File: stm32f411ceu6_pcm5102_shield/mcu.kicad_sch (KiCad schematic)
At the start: 25 parts, among them J100 Conn_01x04_Pin, J101 Conn_01x04_Pin, SW100 RotaryEncoder_Switch_MP, U100 BlackPill, U101 INMP411

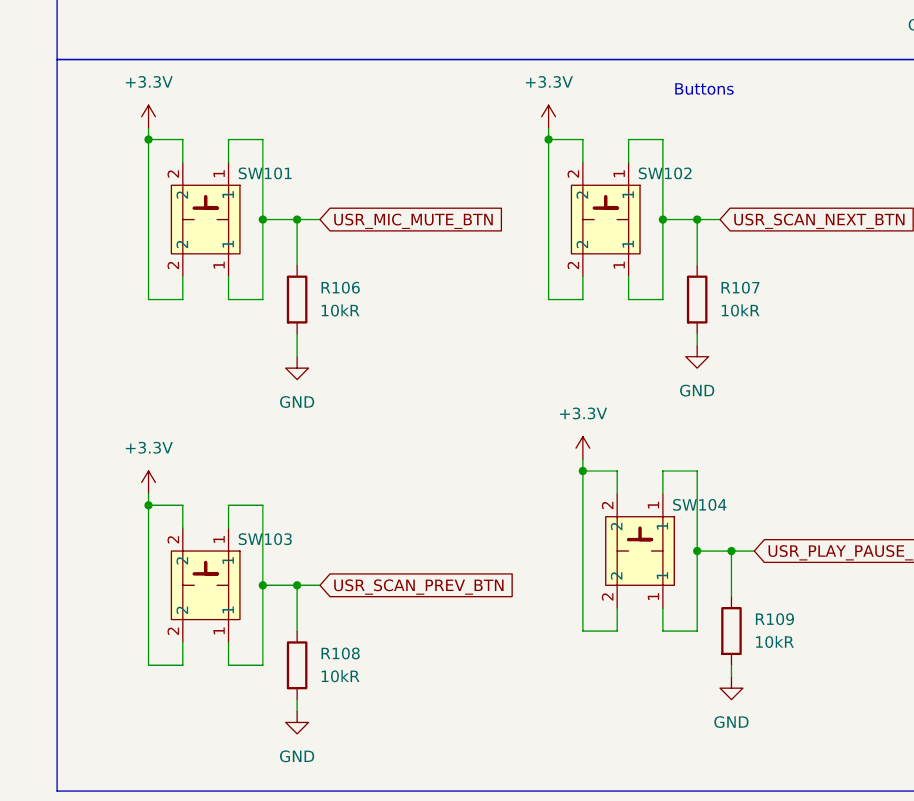
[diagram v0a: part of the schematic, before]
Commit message: Put all items on a board
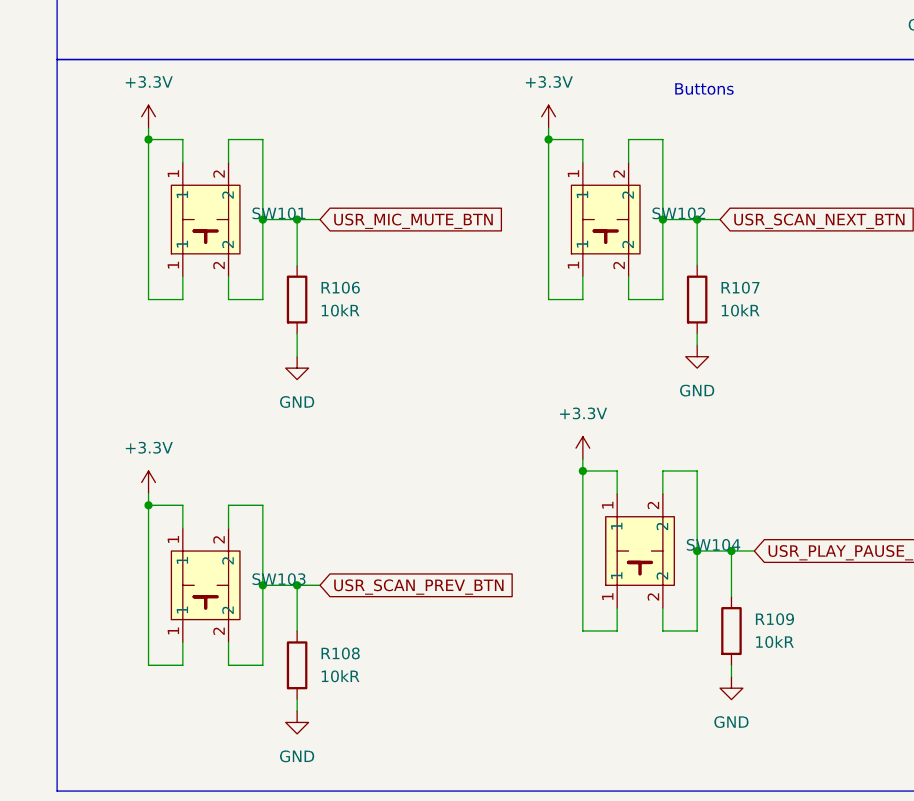
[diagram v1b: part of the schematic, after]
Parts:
- removed SW101, SW102, SW103, SW104: ~, Button_Switch_THT:SW_PUSH_6mm, symbol BlackPillLibrary:SW_PUSH_6mm_H5mm
- added SW101, SW102, SW103, SW104: ~, stm32f401_pcm5102_shiled_lib:SW_PUSH_6mm_H5mm, symbol stm32f401_pcm5102_shiled_lib:SW_PUSH_6mm_H5mm
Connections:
- net +3.3V: now also SW101.1, SW102.1, SW103.1, SW104.1
- net USR_MIC_MUTE_BTN: now also SW101.2
- net USR_PLAY_PAUSE_BTN: now also SW104.2
- net USR_SCAN_NEXT_BTN: now also SW102.2
- net USR_SCAN_PREV_BTN: now also SW103.2

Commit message: PCB rules setup
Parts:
- C100, C101, C102: footprint Capacitor_SMD:C_0805_2012Metric -> Capacitor_SMD:C_0402_1005Metric; Manufacturer Part Number CL21B104KBCNNNC -> CL05B104KO5NNNC
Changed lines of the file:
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@@
 			)
 		)
-		(property "Footprint" "Capacitor_SMD:C_0805_2012Metric"
+		(property "Footprint" "Capacitor_SMD:C_0402_1005Metric"
 			(at 181.3052 48.26 0)
 			(effects
@@
 			)
 		)
-		(property "Manufacturer Part Number" "CL21B104KBCNNNC"
+		(property "Manufacturer Part Number" "CL05B104KO5NNNC"
 			(at 180.34 44.45 0)
 			(effects
@@
 			)
 		)
-		(property "Footprint" "Capacitor_SMD:C_0805_2012Metric"
+		(property "Footprint" "Capacitor_SMD:C_0402_1005Metric"
 			(at 251.1552 54.61 0)
 			(effects
@@
 			)
 		)
-		(property "Manufacturer Part Number" "CL21B104KBCNNNC"
+		(property "Manufacturer Part Number" "CL05B104KO5NNNC"
 			(at 250.19 50.8 0)
 			(effects
@@
 			)
 		)
-		(property "Footprint" "Capacitor_SMD:C_0805_2012Metric"
+		(property "Footprint" "Capacitor_SMD:C_0402_1005Metric"
 			(at 263.8552 54.61 0)
 			(effects
@@
 			)
 		)
-		(property "Manufacturer Part Number" "CL21B104KBCNNNC"
+		(property "Manufacturer Part Number" "CL05B104KO5NNNC"
 			(at 262.89 50.8 0)
 			(effects

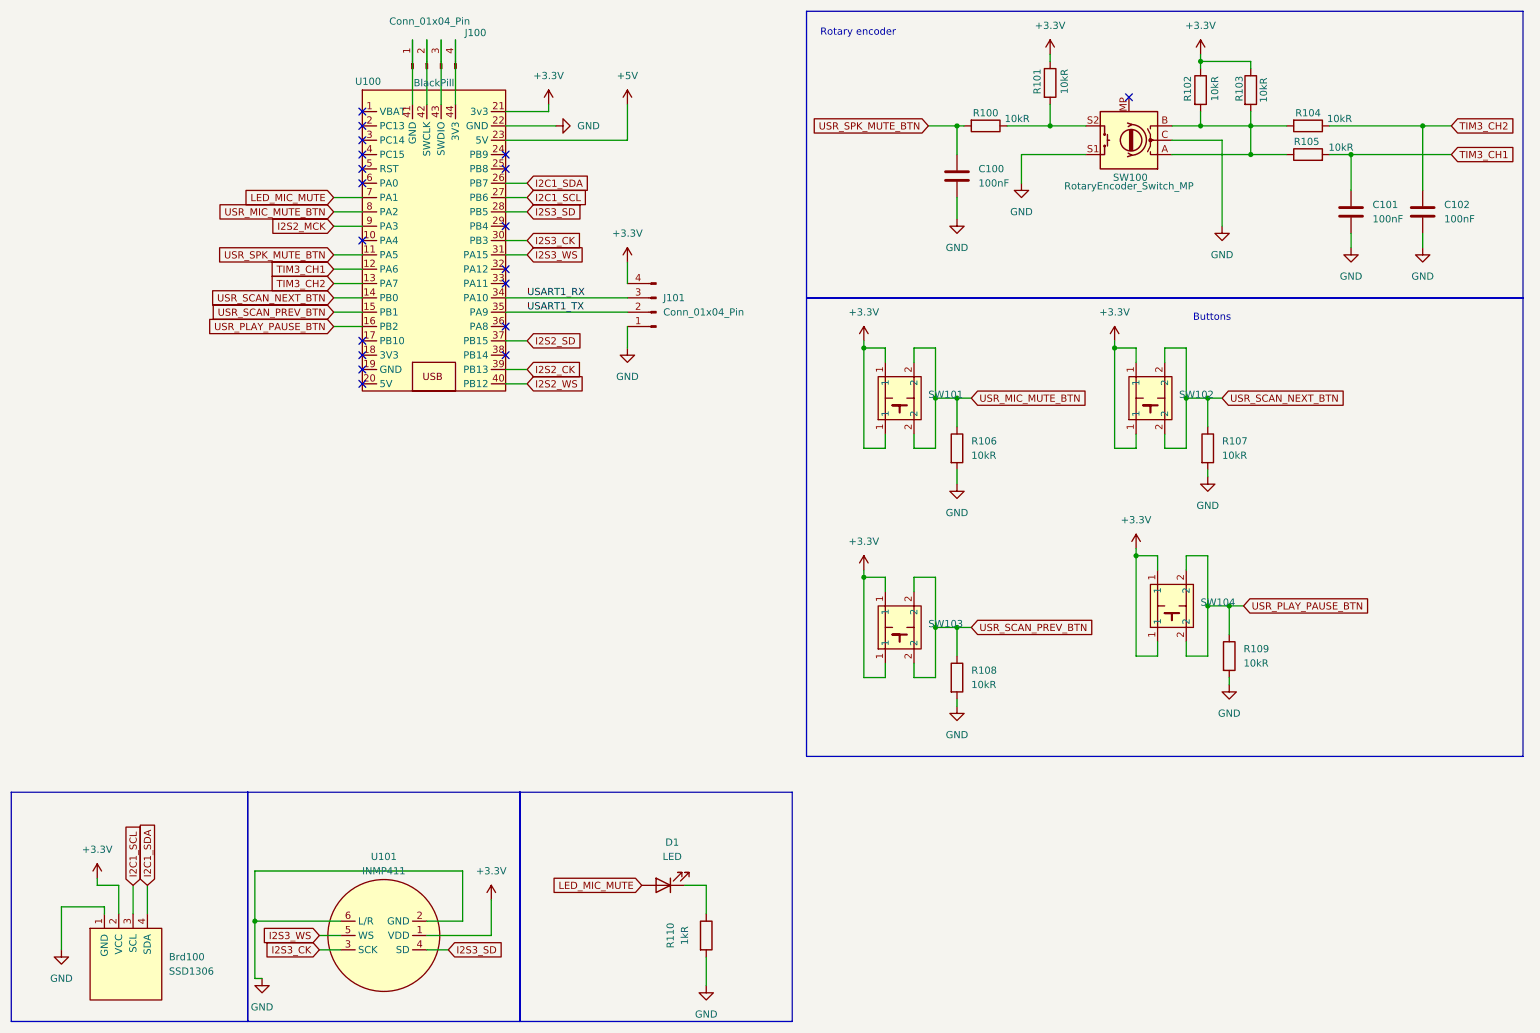
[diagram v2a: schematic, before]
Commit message: Initial layout
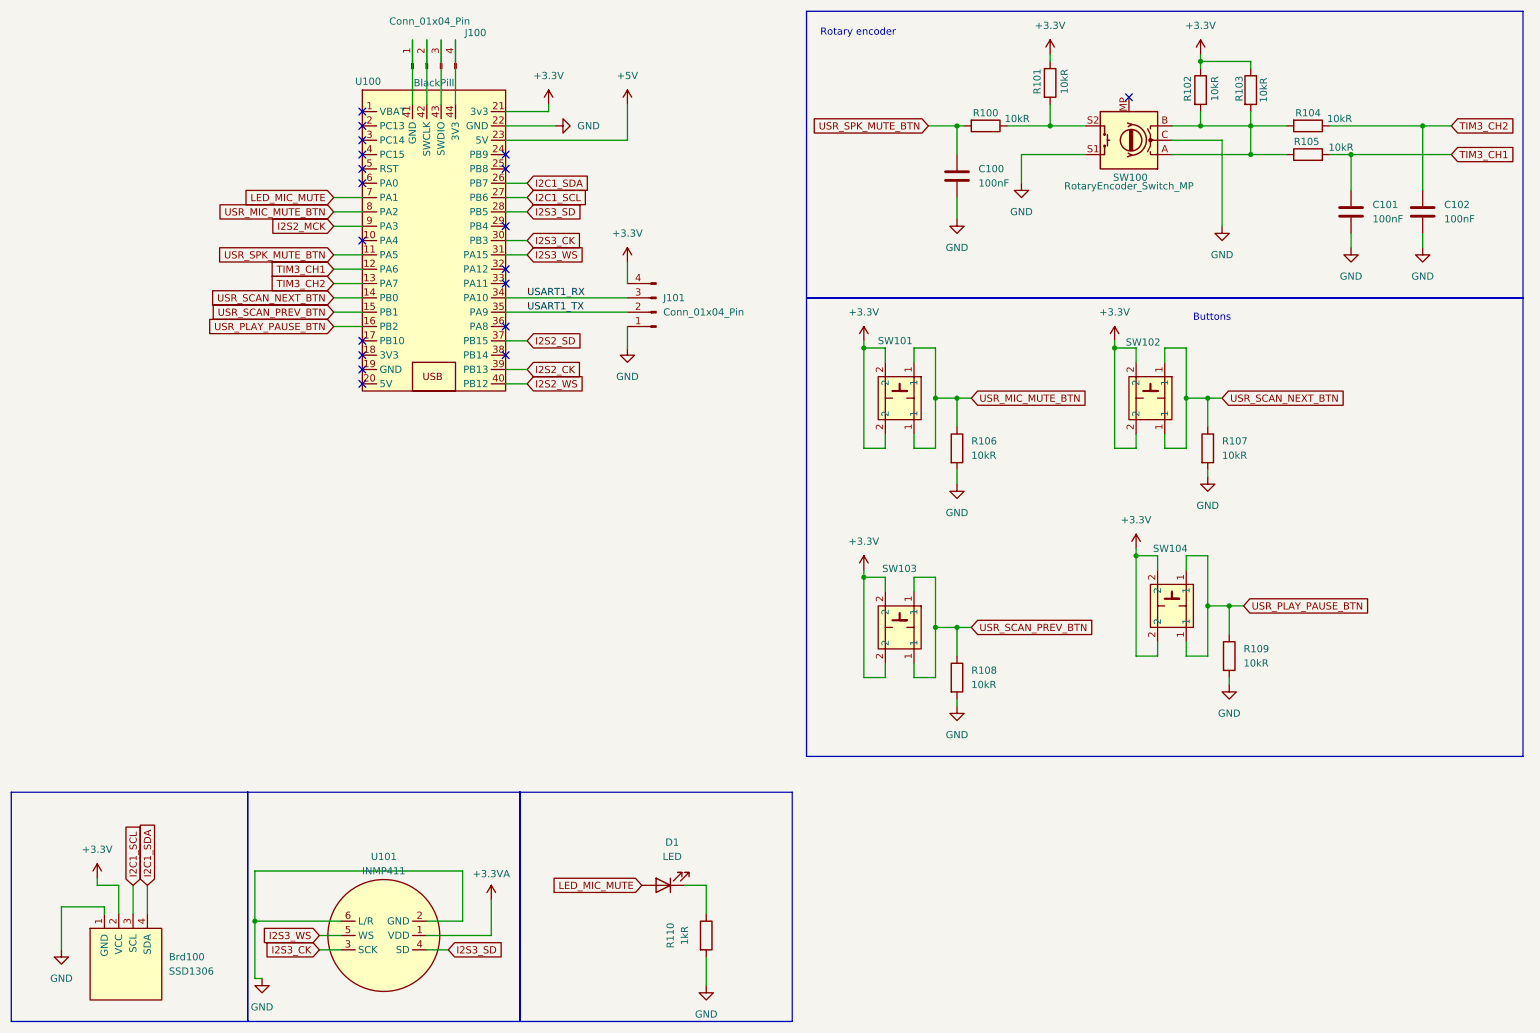
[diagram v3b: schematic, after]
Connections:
- net +3.3V: now also SW101.2, SW102.2, SW103.2, SW104.2; no longer SW101.1, SW102.1, SW103.1, SW104.1, U101.1 (VDD)
- net USR_MIC_MUTE_BTN: now also SW101.1; no longer SW101.2
- net USR_PLAY_PAUSE_BTN: now also SW104.1; no longer SW104.2
- net USR_SCAN_NEXT_BTN: now also SW102.1; no longer SW102.2
- net USR_SCAN_PREV_BTN: now also SW103.1; no longer SW103.2
- new net +3.3VA: U101.1 (VDD)
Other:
- moved on the sheet: SW101, SW102, SW103, SW104
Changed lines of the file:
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@@
+	)
+	(symbol
+		(lib_id "power:+3.3VA")
+		(at 97.79 172.72 0)
+		(unit 1)
+		(exclude_from_sim no)
+		(in_bom yes)
+		(on_board yes)
+		(dnp no)
+		(property "Reference" "#PWR058"
+			(at 97.79 176.53 0)
+			(effects
+				(font
+					(size 1.27 1.27)
+				)
+				(hide yes)
+			)
+		)
+		(property "Value" "+3.3VA"
+			(at 97.79 168.148 0)
+			(effects
+				(font
+					(size 1.27 1.27)
+				)
+			)
+		)
+		(property "Footprint" ""
+			(at 97.79 172.72 0)
+			(effects
+				(font
+					(size 1.27 1.27)
+				)
+				(hide yes)
+			)
+		)
+		(property "Datasheet" ""
+			(at 97.79 172.72 0)
+			(effects
+				(font
+					(size 1.27 1.27)
+				)
+				(hide yes)
+			)
+		)
+		(property "Description" "Power symbol creates a global label with name \"+3.3VA\""
+			(at 97.79 172.72 0)
+			(effects
+				(font
+					(size 1.27 1.27)
+				)
+				(hide yes)
+			)
+		)
+		(pin "1"
+		)
+		(instances
+			(project "stm32f411ceu6_pcm5102_shield"
+				(path "/aeaad843-2b7c-40e9-bb1d-8d1f5e5d5206/850fb9da-5125-4af4-b1b4-d624ecc42efc"
+					(reference "#PWR058")
+					(unit 1)
+				)
+			)
+		)
 	)
 	(symbol
@@
 		(lib_name "stm32f401_pcm5102_shiled_lib:SW_PUSH_6mm_H5mm")
 		(lib_id "stm32f401_pcm5102_shiled_lib:SW_PUSH_6mm_H5mm")
-		(at 168.91 83.82 90)
-		(unit 1)
-		(exclude_from_sim no)
-		(in_bom yes)
-		(on_board yes)
-		(dnp no)
-		(fields_autoplaced yes)
+		(at 171.45 83.82 270)
+		(unit 1)
+		(exclude_from_sim no)
+		(in_bom yes)
+		(on_board yes)
+		(dnp no)
 		(property "Reference" "SW101"
-			(at 175.26 83.1849 90)
+			(at 172.466 73.66 90)
 			(effects
 				(font
@@
 		)
 		(property "Value" "~"
-			(at 175.26 85.09 90)
-			(effects
-				(font
-					(size 1.27 1.27)
-				)
-				(justify right)
+			(at 171.45 83.82 0)
+			(effects
+				(font
+					(size 1.27 1.27)
+				)
 			)
 		)
 		(property "Footprint" "stm32f401_pcm5102_shiled_lib:SW_PUSH_6mm_H5mm"
-			(at 175.768 84.074 0)
+			(at 164.592 83.566 0)
 			(effects
 				(font
@@
 		)
 		(property "Datasheet" ""
-			(at 168.91 83.82 0)
+			(at 171.45 83.82 0)
 			(effects
 				(font
@@
 		)
 		(property "Description" ""
-			(at 168.91 83.82 0)
+			(at 171.45 83.82 0)
 			(effects
 				(font
@@
 		(lib_name "stm32f401_pcm5102_shiled_lib:SW_PUSH_6mm_H5mm")
 		(lib_id "stm32f401_pcm5102_shiled_lib:SW_PUSH_6mm_H5mm")
-		(at 168.91 124.46 90)
-		(unit 1)
-		(exclude_from_sim no)
-		(in_bom yes)
-		(on_board yes)
-		(dnp no)
-		(fields_autoplaced yes)
+		(at 171.45 124.46 270)
+		(unit 1)
+		(exclude_from_sim no)
+		(in_bom yes)
+		(on_board yes)
+		(dnp no)
 		(property "Reference" "SW103"
-			(at 175.26 123.8249 90)
+			(at 173.228 114.046 90)
 			(effects
 				(font
@@
 		)
 		(property "Value" "~"
-			(at 175.26 125.73 90)
-			(effects
-				(font
-					(size 1.27 1.27)
-				)
-				(justify right)
+			(at 171.45 124.46 0)
+			(effects
+				(font
+					(size 1.27 1.27)
+				)
 			)
 		)
 		(property "Footprint" "stm32f401_pcm5102_shiled_lib:SW_PUSH_6mm_H5mm"
-			(at 175.768 124.714 0)
+			(at 164.592 124.206 0)
 			(effects
 				(font
@@
 		)
 		(property "Datasheet" ""
-			(at 168.91 124.46 0)
+			(at 171.45 124.46 0)
 			(effects
 				(font
@@
 		)
 		(property "Description" ""
-			(at 168.91 124.46 0)
+			(at 171.45 124.46 0)
 			(effects
 				(font
@@
 		(lib_name "stm32f401_pcm5102_shiled_lib:SW_PUSH_6mm_H5mm")
 		(lib_id "stm32f401_pcm5102_shiled_lib:SW_PUSH_6mm_H5mm")
-		(at 213.36 83.82 90)
-		(unit 1)
-		(exclude_from_sim no)
-		(in_bom yes)
-		(on_board yes)
-		(dnp no)
-		(fields_autoplaced yes)
+		(at 215.9 83.82 270)
+		(unit 1)
+		(exclude_from_sim no)
+		(in_bom yes)
+		(on_board yes)
+		(dnp no)
 		(property "Reference" "SW102"
-			(at 219.71 83.1849 90)
+			(at 216.408 73.914 90)
 			(effects
 				(font
@@
 		)
 		(property "Value" "~"
-			(at 219.71 85.09 90)
-			(effects
-				(font
-					(size 1.27 1.27)
-				)
-				(justify right)
+			(at 215.9 83.82 0)
+			(effects
+				(font
+					(size 1.27 1.27)
+				)
 			)
 		)
 		(property "Footprint" "stm32f401_pcm5102_shiled_lib:SW_PUSH_6mm_H5mm"
-			(at 220.218 84.074 0)
+			(at 209.042 83.566 0)
 			(effects
 				(font
@@
 		)
 		(property "Datasheet" ""
-			(at 213.36 83.82 0)
+			(at 215.9 83.82 0)
 			(effects
 				(font
@@
 		)
 		(property "Description" ""
-			(at 213.36 83.82 0)
+			(at 215.9 83.82 0)
 			(effects
 				(font
@@
 	)
 	(symbol
-		(lib_id "power:+3.3V")
-		(at 97.79 172.72 0)
-		(unit 1)
-		(exclude_from_sim no)
-		(in_bom yes)
-		(on_board yes)
-		(dnp no)
-		(fields_autoplaced yes)
-		(property "Reference" "#PWR058"
-			(at 97.79 176.53 0)
-			(effects
-				(font
-					(size 1.27 1.27)
-				)
-				(hide yes)
-			)
-		)
-		(property "Value" "+3.3V"
-			(at 97.79 167.64 0)
-			(effects
-				(font
-					(size 1.27 1.27)
-				)
-			)
-		)
-		(property "Footprint" ""
-			(at 97.79 172.72 0)
-			(effects
-				(font
-					(size 1.27 1.27)
-				)
-				(hide yes)
-			)
-		)
-		(property "Datasheet" ""
-			(at 97.79 172.72 0)
-			(effects
-				(font
-					(size 1.27 1.27)
-				)
-				(hide yes)
-			)
-		)
-		(property "Description" "Power symbol creates a global label with name \"+3.3V\""
-			(at 97.79 172.72 0)
-			(effects
-				(font
-					(size 1.27 1.27)
-				)
-				(hide yes)
-			)
-		)
-		(pin "1"
-		)
-		(instances
-			(project "stm32f411ceu6_pcm5102_shield"
-				(path "/aeaad843-2b7c-40e9-bb1d-8d1f5e5d5206/850fb9da-5125-4af4-b1b4-d624ecc42efc"
-					(reference "#PWR058")
-					(unit 1)
-				)
-			)
-		)
-	)
-	(symbol
 		(lib_id "power:GND")
 		(at 228.6 134.62 0)
@@
 		(lib_name "stm32f401_pcm5102_shiled_lib:SW_PUSH_6mm_H5mm")
 		(lib_id "stm32f401_pcm5102_shiled_lib:SW_PUSH_6mm_H5mm")
-		(at 217.17 120.65 90)
-		(unit 1)
-		(exclude_from_sim no)
-		(in_bom yes)
-		(on_board yes)
-		(dnp no)
-		(fields_autoplaced yes)
+		(at 219.71 120.65 270)
+		(unit 1)
+		(exclude_from_sim no)
+		(in_bom yes)
+		(on_board yes)
+		(dnp no)
 		(property "Reference" "SW104"
-			(at 223.52 120.0149 90)
+			(at 221.234 110.49 90)
 			(effects
 				(font
@@
 		)
 		(property "Value" "~"
-			(at 223.52 121.92 90)
-			(effects
-				(font
-					(size 1.27 1.27)
-				)
-				(justify right)
+			(at 219.71 120.65 0)
+			(effects
+				(font
+					(size 1.27 1.27)
+				)
 			)
 		)
 		(property "Footprint" "stm32f401_pcm5102_shiled_lib:SW_PUSH_6mm_H5mm"
-			(at 224.028 120.904 0)
+			(at 212.852 120.396 0)
 			(effects
 				(font
@@
 		)
 		(property "Datasheet" ""
-			(at 217.17 120.65 0)
+			(at 219.71 120.65 0)
 			(effects
 				(font
@@
 		)
 		(property "Description" ""
-			(at 217.17 120.65 0)
-			(effects
-				(font
+			(at 219.71 120.65 0)
+			(effects
+				(font
